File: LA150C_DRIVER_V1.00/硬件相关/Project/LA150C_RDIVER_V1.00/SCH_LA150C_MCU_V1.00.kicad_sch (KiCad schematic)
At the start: 14 parts, among them U1 GD32F503REL7, X1 CSTCE8M00G52-R0

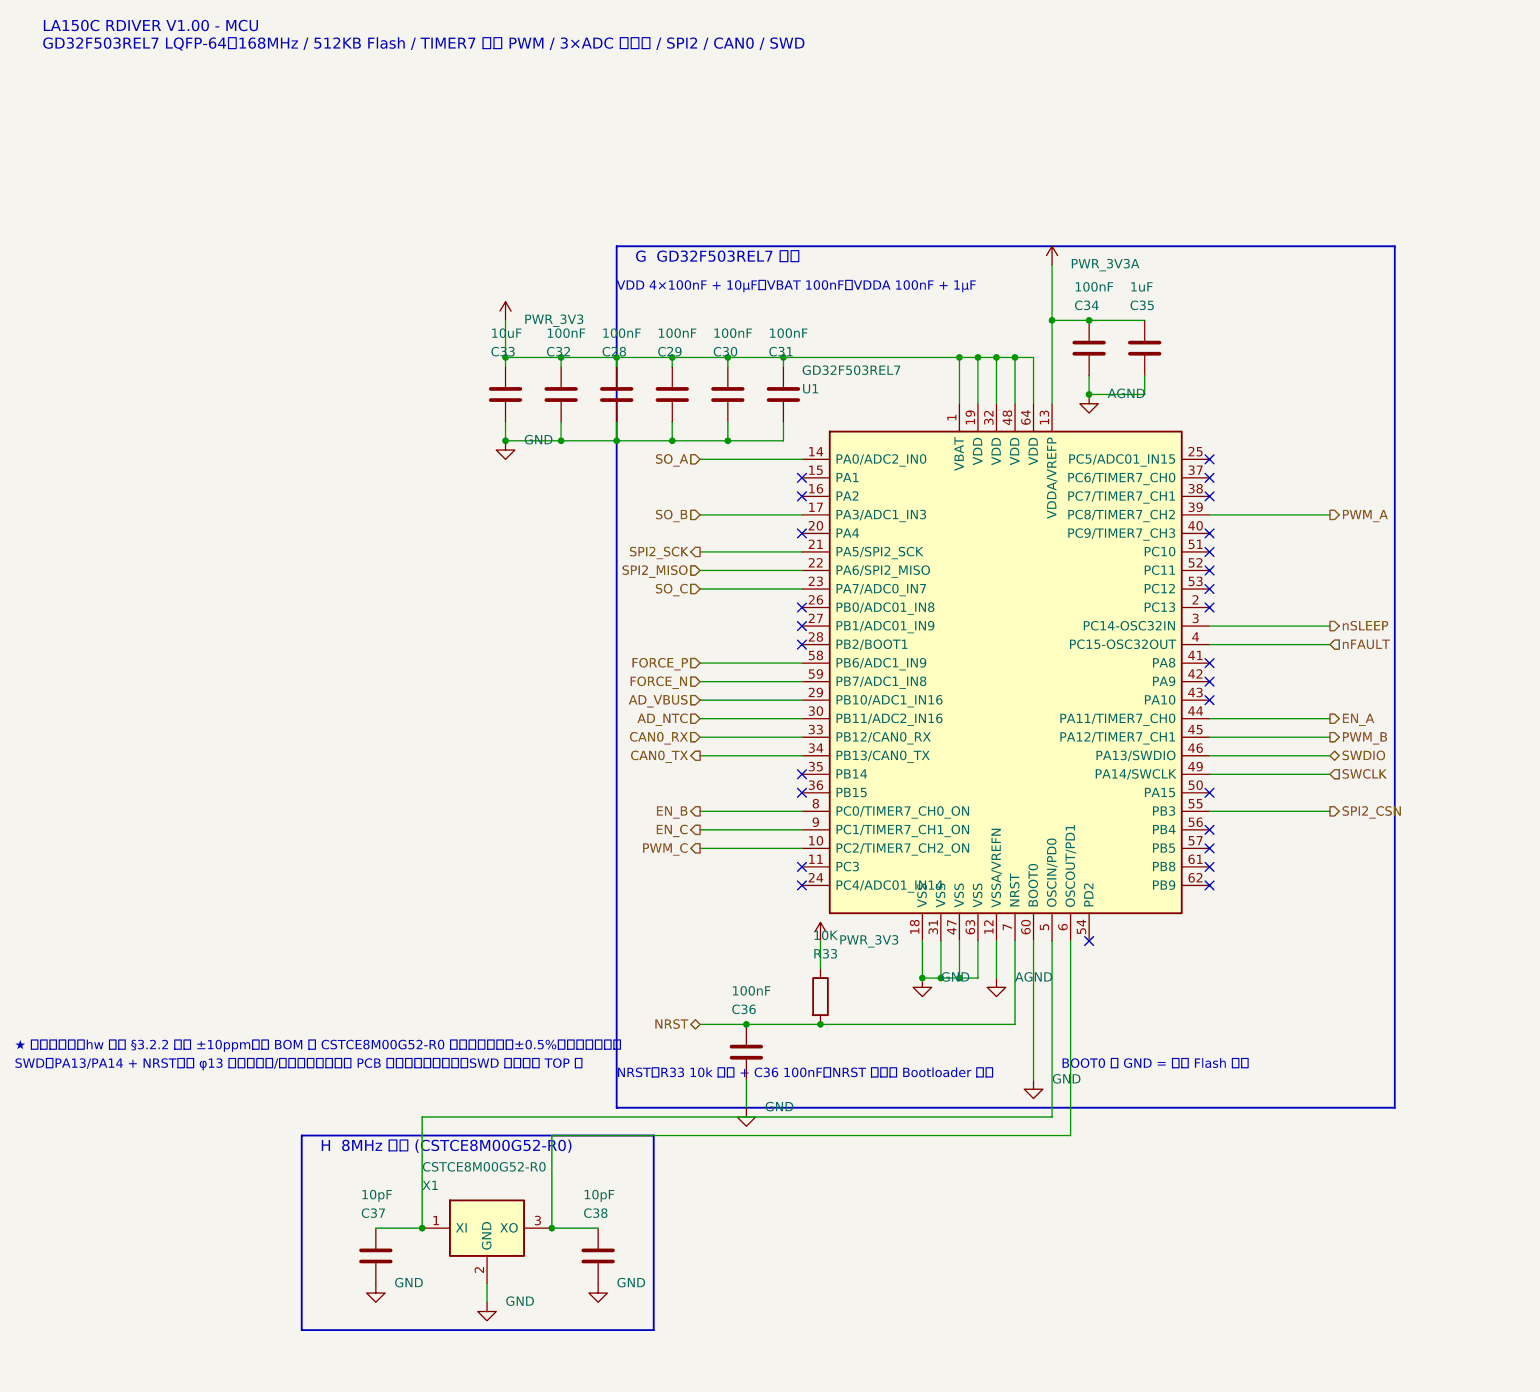
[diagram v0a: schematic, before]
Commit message: chore: save LA150C schematic updates
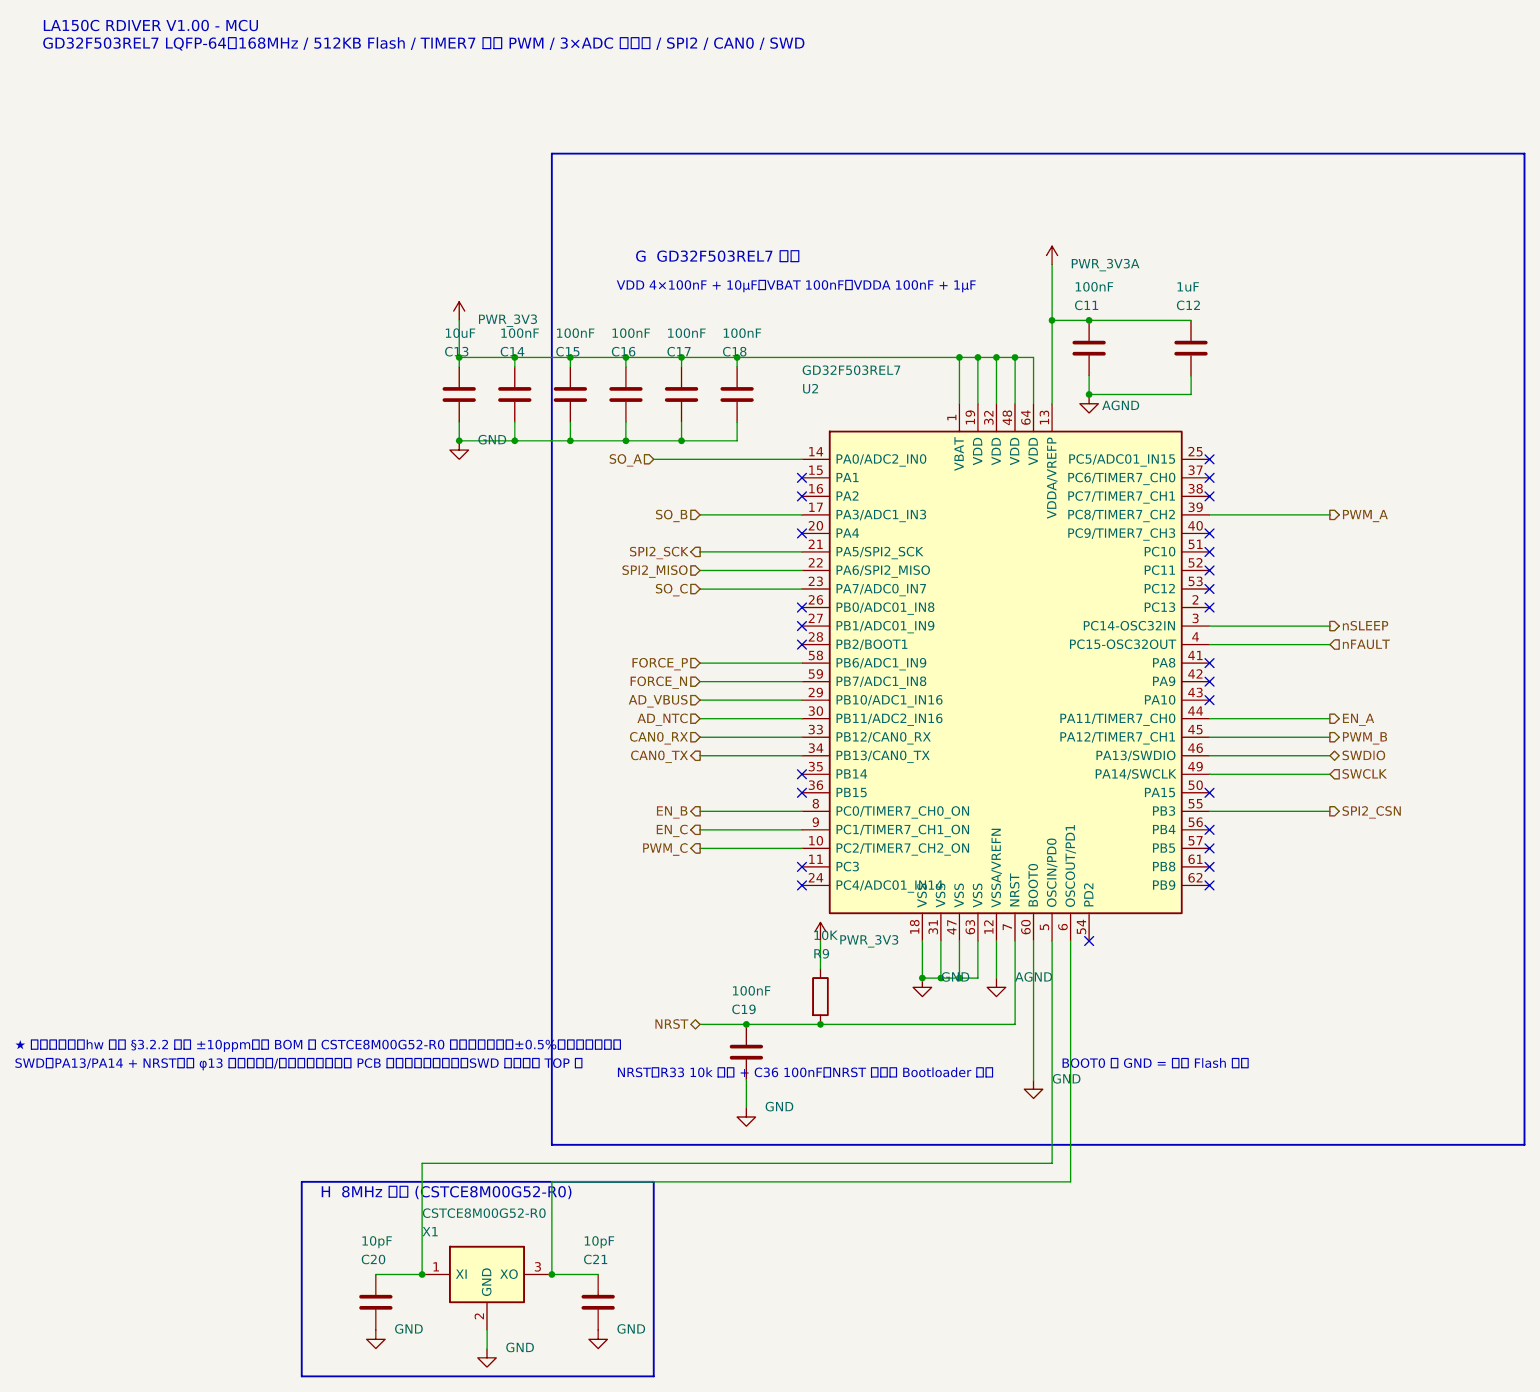
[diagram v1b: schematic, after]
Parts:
- renumbered C34 to C11, C35 to C12, C33 to C13, C32 to C14, C28 to C15, C29 to C16, C30 to C17, C31 to C18, C36 to C19, C37 to C20, C38 to C21, R33 to R9, U1 to U2
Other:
- moved on the sheet: C12, C13, C14, C15, C16, C17, C18, C20, C21, X1
